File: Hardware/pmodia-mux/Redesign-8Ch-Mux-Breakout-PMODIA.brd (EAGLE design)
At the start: 26.1 x 66.1 mm, 32 parts, among them U1 74HC4051BQ, U2 74HC4051BQ, U3 AD5933, U4 AD8606, U5 ADP150, U6 AD8606

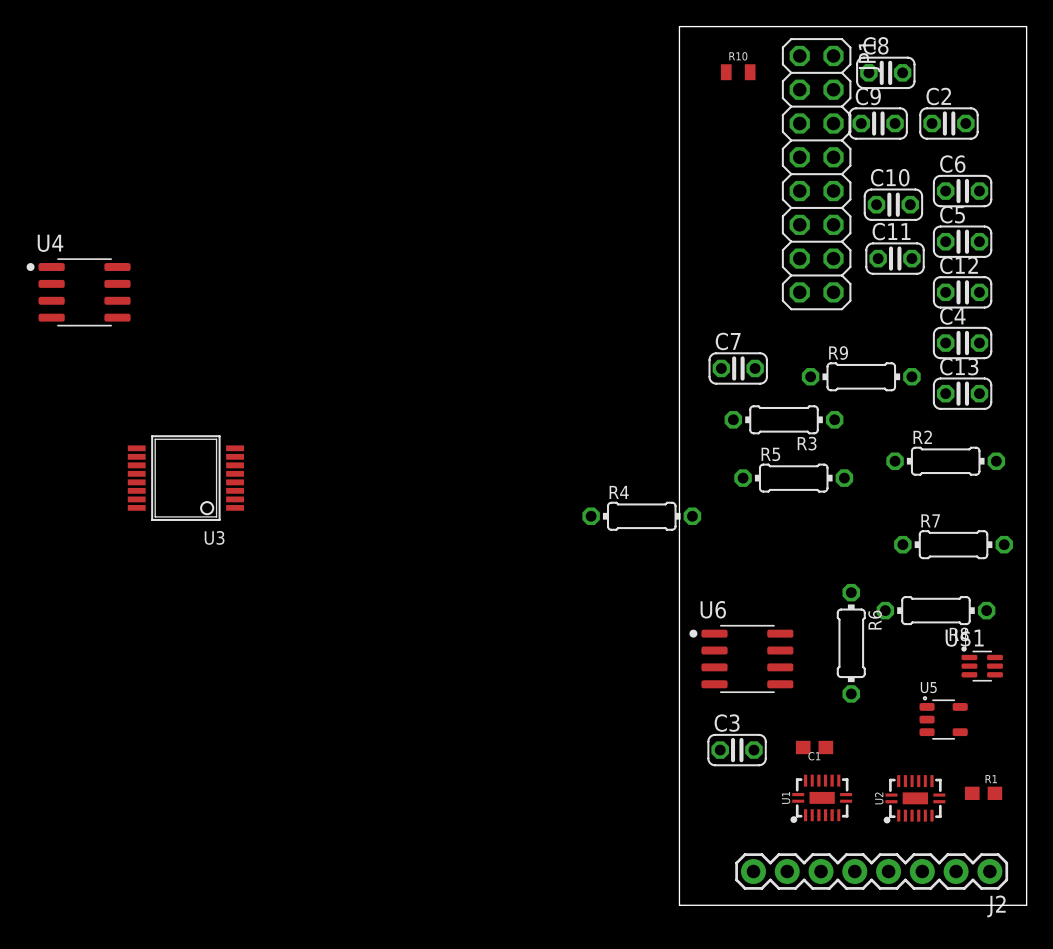
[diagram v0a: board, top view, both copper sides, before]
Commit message: Add files via upload
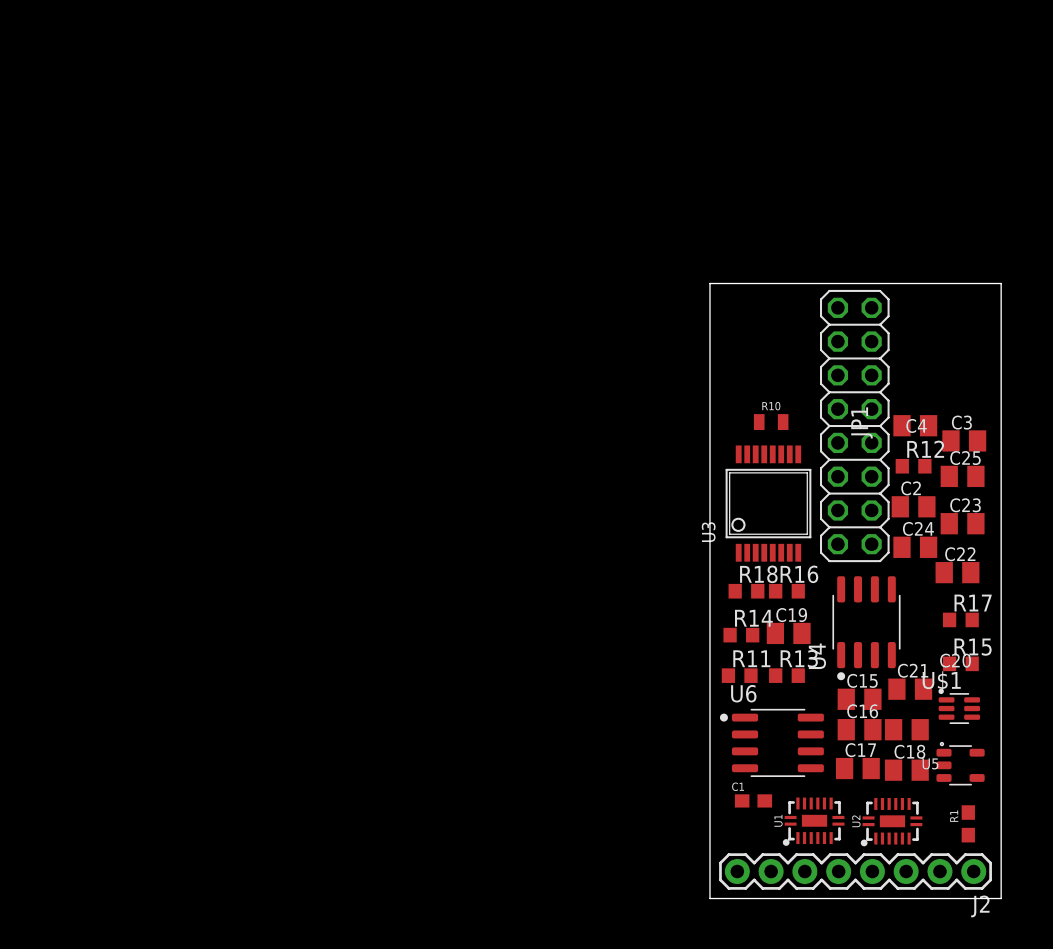
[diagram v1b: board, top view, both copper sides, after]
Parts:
- removed C10, C11, C8, C9: (no value), rcl:C025-024X044
- removed C12: 10uF, rcl:C025-024X044
- removed C13, C5, C6: 0.1uF, rcl:C025-024X044
- removed C7: 47nF, rcl:C025-024X044
- removed R2, R3, R6, R7: 49.9K, rcl:0204/7
- removed R4: 20K, rcl:0204/7
- removed R5: (no value), rcl:0204/7
- removed R8: 20, rcl:0204/7
- removed R9: 100K, rcl:0204/7
- added C15, C16, C20, C22, C25: 10uF, rcl:C0805K
- added C17, C18, C21, C23, C24: 0.1uF, rcl:C0805K
- added C19: 47nF, rcl:C0805K
- added R11, R12, R13, R14: 49.9K, rcl:R0603
- added R15: 20, rcl:R0603
- added R16, R18: 20K, rcl:R0603
- added R17: 100K, rcl:R0603
- C2, C4: value 10uF -> 0.1uF; device rcl:C025-024X044 -> rcl:C0805K
- C3: value 0.1uF -> 10uF; device rcl:C025-024X044 -> rcl:C0805K
- moved U4 63.8 mm to (16.9, 6.94), turned to 90 degrees
- moved U3 43.9 mm to (9.53, 15.9), turned to 0 degrees
- moved C2 29.0 mm to (20.4, 15.6)
- moved C3 28.9 mm to (24.3, 20.6)
- moved R10 26.4 mm to (9.73, 22.0)
- moved JP1 19.2 mm to (16.0, 21.7)
- moved C4 7.17 mm to (20.6, 21.7)
- moved U6 6.72 mm to (10.2, -2.14)
- moved C1 6.10 mm to (8.40, -6.50)
- moved U5 3.67 mm to (24.0, -3.83)
- moved U$1 3.63 mm to (23.9, 0.45)
- moved R1 2.57 mm to (24.6, -8.22), turned to 90 degrees
- moved U2 2.44 mm to (18.9, -8.03)
- moved U1 1.82 mm to (13.0, -8.00)
- moved J2 1.21 mm to (25.0, -11.8)
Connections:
- net GND: now also C15.2, C16.2, C17.2, C18.2, C20.2, C21.2, C22.2, C23.1, C24.2, C25.2, R11.2, R14.1, U6.4; no longer C10.2, C11.2, C12.2, C13.2, C5.2, C6.2, C8.2, C9.2, R2.2, R7.1, U6.8
- net N$1: now also C19.1; no longer C7.1
- net N$11: now also R16.1; no longer R5.2
- net N$3: now also C19.2, R11.1, R12.2; no longer C7.2, R2.1, R3.2
- net N$4: now also R13.1, R14.2; no longer R6.1, R7.2
- net N$5: now also R18.2; no longer R4.2
- net N$6: now also R15.2; no longer R8.1
- net N$9: now also R17.2; no longer R9.1
- net VCC: now also C18.1, C23.2, C25.1, C4.1; no longer C2.1, C6.1, C8.1, C9.1
- net VCC3V0: now also C15.1, C16.1, C17.1, C2.1, C20.1, C21.1, C22.1, C24.1, R12.1, R13.2, U6.8; no longer C10.1, C11.1, C12.1, C13.1, C4.1, C5.1, R3.1, R6.2, U6.4
- net VIN: now also R16.2, R18.1; no longer R4.1, R5.1
- net Z2: now also R15.1, R17.1; no longer R8.2, R9.2
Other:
- board size 26.1 x 66.1 mm -> 21.9 x 46.3 mm
